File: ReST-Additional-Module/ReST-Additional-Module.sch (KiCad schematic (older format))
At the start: 11 parts, among them P1 CONN_02X06, P2 02-SCREW-TERM, P3 02-SCREW-TERM, Q1 Q_BSH105, Q2 Q_AOT240L

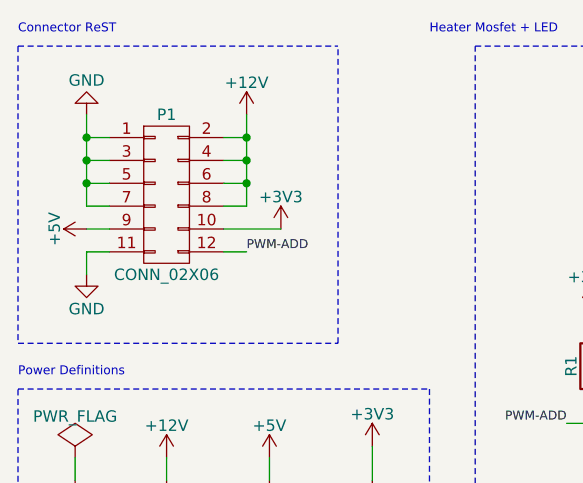
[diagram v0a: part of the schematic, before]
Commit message: Saving
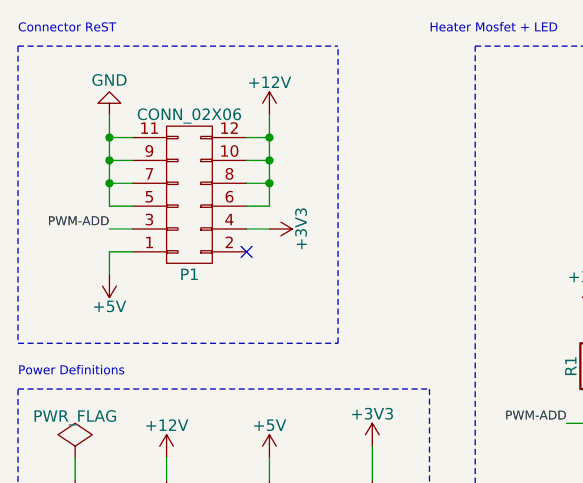
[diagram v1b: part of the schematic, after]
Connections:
- net +12V: now also P1.10 (P10), P1.12 (P12); no longer P1.2 (P2), P1.4 (P4)
- net +3V3: now also P1.4 (P4); no longer P1.10 (P10)
- net +5V: now also P1.1 (P1); no longer P1.9 (P9)
- net GND: now also P1.9 (P9); no longer P1.1 (P1), P1.3 (P3)
- net PWM-ADD: now also P1.3 (P3); no longer P1.12 (P12)
- no-connect marks 0 -> 1
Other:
- moved on the sheet: P1
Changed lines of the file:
@@
 L +5V #PWR02
 U 1 1 56A6A1BB
-P 2950 2900
-F 0 "#PWR02" H 2950 2750 50  0001 C CNN
-F 1 "+5V" H 2950 3040 50  0000 C CNN
-F 2 "" H 2950 2900 50  0000 C CNN
-F 3 "" H 2950 2900 50  0000 C CNN
-	1    2950 2900
-	0    -1   -1   0
+P 3050 3100
+F 0 "#PWR02" H 3050 2950 50  0001 C CNN
+F 1 "+5V" H 3050 3240 50  0000 C CNN
+F 2 "" H 3050 3100 50  0000 C CNN
+F 3 "" H 3050 3100 50  0000 C CNN
+	1    3050 3100
+	-1   0    0    1
 $EndComp
 $Comp
 L +3V3 #PWR03
 U 1 1 56A6A1DD
-P 3800 2900
-F 0 "#PWR03" H 3800 2750 50  0001 C CNN
-F 1 "+3V3" H 3800 3040 50  0000 C CNN
-F 2 "" H 3800 2900 50  0000 C CNN
-F 3 "" H 3800 2900 50  0000 C CNN
-	1    3800 2900
-	1    0    0    -1
+P 3750 2900
+F 0 "#PWR03" H 3750 2750 50  0001 C CNN
+F 1 "+3V3" H 3750 3040 50  0000 C CNN
+F 2 "" H 3750 2900 50  0000 C CNN
+F 3 "" H 3750 2900 50  0000 C CNN
+	1    3750 2900
+	0    1    1    0
 $EndComp
 $Comp
 L GND #PWR04
-U 1 1 56A6A1FF
-P 2950 3100
-F 0 "#PWR04" H 2950 2850 50  0001 C CNN
-F 1 "GND" H 2950 2950 50  0000 C CNN
-F 2 "" H 2950 3100 50  0000 C CNN
-F 3 "" H 2950 3100 50  0000 C CNN
-	1    2950 3100
-	1    0    0    -1
-$EndComp
-$Comp
-L GND #PWR05
 U 1 1 56A6B6EF
 P 6850 3850
-F 0 "#PWR05" H 6850 3600 50  0001 C CNN
+F 0 "#PWR04" H 6850 3600 50  0001 C CNN
 F 1 "GND" H 6850 3700 50  0000 C CNN
 F 2 "" H 6850 3850 50  0000 C CNN
@@
 $EndComp
 $Comp
-L +3V3 #PWR06
+L +3V3 #PWR05
 U 1 1 56A6D2B8
 P 5150 3250
-F 0 "#PWR06" H 5150 3100 50  0001 C CNN
+F 0 "#PWR05" H 5150 3100 50  0001 C CNN
 F 1 "+3V3" H 5150 3390 50  0000 C CNN
 F 2 "" H 5150 3250 50  0000 C CNN
@@
 $EndComp
 $Comp
-L +5V #PWR07
+L +5V #PWR06
 U 1 1 56A6D350
 P 5550 2750
-F 0 "#PWR07" H 5550 2600 50  0001 C CNN
+F 0 "#PWR06" H 5550 2600 50  0001 C CNN
 F 1 "+5V" H 5550 2890 50  0000 C CNN
 F 2 "" H 5550 2750 50  0000 C CNN
@@
 $EndComp
 $Comp
-L GND #PWR08
+L GND #PWR07
 U 1 1 56A6DF02
 P 5550 4050
-F 0 "#PWR08" H 5550 3800 50  0001 C CNN
+F 0 "#PWR07" H 5550 3800 50  0001 C CNN
 F 1 "GND" H 5550 3900 50  0000 C CNN
 F 2 "" H 5550 4050 50  0000 C CNN
@@
 Text Label 5050 3750 2    39   ~ 0
 PWM-ADD
-Text Label 3650 3000 0    39   ~ 0
+Text Label 3050 2900 2    39   ~ 0
 PWM-ADD
 $Comp
-L +12V #PWR09
+L +12V #PWR08
 U 1 1 56A7EB7B
 P 3300 3900
-F 0 "#PWR09" H 3300 3750 50  0001 C CNN
+F 0 "#PWR08" H 3300 3750 50  0001 C CNN
 F 1 "+12V" H 3300 4040 50  0000 C CNN
 F 2 "" H 3300 3900 50  0000 C CNN
@@
 $EndComp
 $Comp
-L GND #PWR010
+L GND #PWR09
 U 1 1 56A7EBB6
 P 2900 4000
-F 0 "#PWR010" H 2900 3750 50  0001 C CNN
+F 0 "#PWR09" H 2900 3750 50  0001 C CNN
 F 1 "GND" H 2900 3850 50  0000 C CNN
 F 2 "" H 2900 4000 50  0000 C CNN
@@
 $EndComp
 $Comp
-L +5V #PWR011
+L +5V #PWR010
 U 1 1 56A7EBF1
 P 3750 3900
-F 0 "#PWR011" H 3750 3750 50  0001 C CNN
+F 0 "#PWR010" H 3750 3750 50  0001 C CNN
 F 1 "+5V" H 3750 4040 50  0000 C CNN
 F 2 "" H 3750 3900 50  0000 C CNN
@@
 $EndComp
 $Comp
-L +3V3 #PWR012
+L +3V3 #PWR011
 U 1 1 56A7EC2C
 P 4200 3850
-F 0 "#PWR012" H 4200 3700 50  0001 C CNN
+F 0 "#PWR011" H 4200 3700 50  0001 C CNN
 F 1 "+3V3" H 4200 3990 50  0000 C CNN
 F 2 "" H 4200 3850 50  0000 C CNN
@@
 $EndComp
 $Comp
-L PWR_FLAG #FLG013
+L PWR_FLAG #FLG012
 U 1 1 56A7EC59
 P 4200 4000
-F 0 "#FLG013" H 4200 4095 50  0001 C CNN
+F 0 "#FLG012" H 4200 4095 50  0001 C CNN
 F 1 "PWR_FLAG" H 4200 4180 50  0000 C CNN
 F 2 "" H 4200 4000 50  0000 C CNN
@@
 $EndComp
 $Comp
-L PWR_FLAG #FLG014
+L PWR_FLAG #FLG013
 U 1 1 56A7EC9B
 P 3750 4000
-F 0 "#FLG014" H 3750 4095 50  0001 C CNN
+F 0 "#FLG013" H 3750 4095 50  0001 C CNN
 F 1 "PWR_FLAG" H 3750 4180 50  0000 C CNN
 F 2 "" H 3750 4000 50  0000 C CNN
@@
 $EndComp
 $Comp
-L PWR_FLAG #FLG015
+L PWR_FLAG #FLG014
 U 1 1 56A7ECD6
 P 3300 4000
-F 0 "#FLG015" H 3300 4095 50  0001 C CNN
+F 0 "#FLG014" H 3300 4095 50  0001 C CNN
 F 1 "PWR_FLAG" H 3300 4180 50  0000 C CNN
 F 2 "" H 3300 4000 50  0000 C CNN
@@
 $EndComp
 $Comp
-L PWR_FLAG #FLG016
+L PWR_FLAG #FLG015
 U 1 1 56A7ED11
 P 2900 3900
-F 0 "#FLG016" H 2900 3995 50  0001 C CNN
+F 0 "#FLG015" H 2900 3995 50  0001 C CNN
 F 1 "PWR_FLAG" H 2900 4080 50  0000 C CNN
 F 2 "" H 2900 3900 50  0000 C CNN
@@
 Power Definitions
 $Comp
-L +12V #PWR017
+L +12V #PWR016
 U 1 1 56AC08E7
-P 3650 2400
-F 0 "#PWR017" H 3650 2250 50  0001 C CNN
-F 1 "+12V" H 3650 2540 50  0000 C CNN
-F 2 "" H 3650 2400 50  0000 C CNN
-F 3 "" H 3650 2400 50  0000 C CNN
-	1    3650 2400
-	1    0    0    -1
-$EndComp
-$Comp
-L GND #PWR018
+P 3750 2400
+F 0 "#PWR016" H 3750 2250 50  0001 C CNN
+F 1 "+12V" H 3750 2540 50  0000 C CNN
+F 2 "" H 3750 2400 50  0000 C CNN
+F 3 "" H 3750 2400 50  0000 C CNN
+	1    3750 2400
+	1    0    0    -1
+$EndComp
+$Comp
+L GND #PWR017
 U 1 1 56AC091C
-P 2950 2400
-F 0 "#PWR018" H 2950 2150 50  0001 C CNN
-F 1 "GND" H 2950 2250 50  0000 C CNN
-F 2 "" H 2950 2400 50  0000 C CNN
-F 3 "" H 2950 2400 50  0000 C CNN
-	1    2950 2400
+P 3050 2400
+F 0 "#PWR017" H 3050 2150 50  0001 C CNN
+F 1 "GND" H 3050 2250 50  0000 C CNN
+F 2 "" H 3050 2400 50  0000 C CNN
+F 3 "" H 3050 2400 50  0000 C CNN
+	1    3050 2400
 	-1   0    0    1
 $EndComp
@@
 L CONN_02X06 P1
 U 1 1 56AD3C5B
-P 3300 2750
-F 0 "P1" H 3300 3100 50  0000 C CNN
-F 1 "CONN_02X06" H 3300 2400 50  0000 C CNN
-F 2 "Pin_Headers:Pin_Header_Angled_2x06" H 3300 1550 50  0001 C CNN
-F 3 "" H 3300 1550 50  0000 C CNN
-	1    3300 2750
-	1    0    0    -1
-$EndComp
-Wire Wire Line
-	3650 2400 3650 2800
-Wire Wire Line
-	3650 2500 3550 2500
-Wire Wire Line
-	3650 2600 3550 2600
-Connection ~ 3650 2500
-Wire Wire Line
-	3650 2700 3550 2700
-Connection ~ 3650 2600
-Wire Wire Line
-	3650 2800 3550 2800
-Connection ~ 3650 2700
-Wire Wire Line
-	2950 2400 2950 2800
-Wire Wire Line
-	2950 2500 3050 2500
-Wire Wire Line
-	2950 2600 3050 2600
-Connection ~ 2950 2500
-Wire Wire Line
-	2950 2700 3050 2700
-Connection ~ 2950 2600
-Wire Wire Line
-	2950 2800 3050 2800
-Connection ~ 2950 2700
-Wire Wire Line
-	2950 2900 3050 2900
-Wire Wire Line
-	3550 2900 3800 2900
-Wire Wire Line
-	3050 3000 2950 3000
-Wire Wire Line
-	2950 3000 2950 3100
-Wire Wire Line
-	3650 3000 3550 3000
+P 3400 2750
+F 0 "P1" H 3400 3100 50  0000 C CNN
+F 1 "CONN_02X06" H 3400 2400 50  0000 C CNN
+F 2 "Pin_Headers:Pin_Header_Angled_2x06" H 3400 1550 50  0001 C CNN
+F 3 "" H 3400 1550 50  0000 C CNN
+	1    3400 2750
+	1    0    0    1
+$EndComp
+Wire Wire Line
+	3750 2400 3750 2800
+Wire Wire Line
+	3750 2500 3650 2500
+Wire Wire Line
+	3750 2600 3650 2600
+Connection ~ 3750 2500
+Wire Wire Line
+	3750 2700 3650 2700
+Connection ~ 3750 2600
+Wire Wire Line
+	3750 2800 3650 2800
+Connection ~ 3750 2700
+Wire Wire Line
+	3050 2400 3050 2800
+Wire Wire Line
+	3050 2500 3150 2500
+Wire Wire Line
+	3050 2600 3150 2600
+Connection ~ 3050 2500
+Wire Wire Line
+	3050 2700 3150 2700
+Connection ~ 3050 2600
+Wire Wire Line
+	3050 2800 3150 2800
+Connection ~ 3050 2700
 Wire Notes Line
 	2650 2100 4050 2100
@@
 Wire Notes Line
 	4050 3400 4050 2100
+Wire Wire Line
+	3750 2900 3650 2900
+Wire Wire Line
+	3150 2900 3050 2900
+Wire Wire Line
+	3050 3100 3050 3000
+Wire Wire Line
+	3050 3000 3150 3000
+NoConn ~ 3650 3000
 $EndSCHEMATC
